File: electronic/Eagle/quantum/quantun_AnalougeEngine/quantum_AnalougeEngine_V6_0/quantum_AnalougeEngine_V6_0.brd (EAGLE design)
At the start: 210 x 70 mm, 281 parts, among them IC1 OP275, IC10 STM32F767ZIT6, IC11 PGA2320IDW, IC12 ESDA6V1BC6, IC13 USBLC6-4SC6, IC16 OP275, IC17 AD7606BSTZ-6, IC2 DAC084S085CIMM_NOPB, IC4 OP275, IC6 LAN8742A-CZ-TR, IC8 OP275, IC9 NE5532, J1 GWLEX-SMT-S988G_Y, K1 Relay, K2 Relay, K3 Relay, K4 Relay, K5 Relay, K6 Relay, K7 Relay, K8 Relay, T1 H1102NL, U1 78*_SMD, U12 ULN2003, U4 THAT1240, U6 THAT1240, U7 THAT1240, U8 THAT1240, Y1 NX3215SA-32.768K-STD-MUA-8, Y2 NX3225GD-8MHZ-STD-CRA-3, Y3 ABLS2-25.000MHZ-D4YF-T

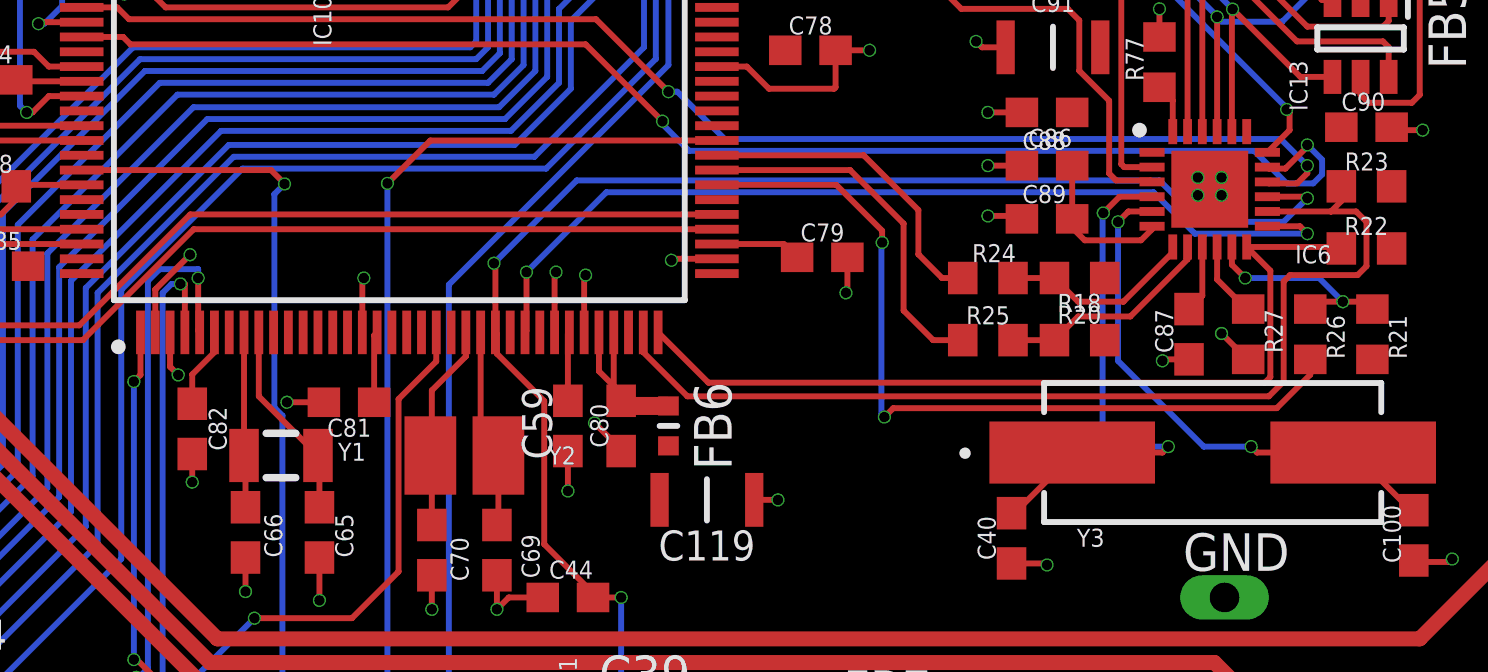
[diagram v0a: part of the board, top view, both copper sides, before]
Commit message: AnaloougeEngine_V6_0 & PSU_V2_3
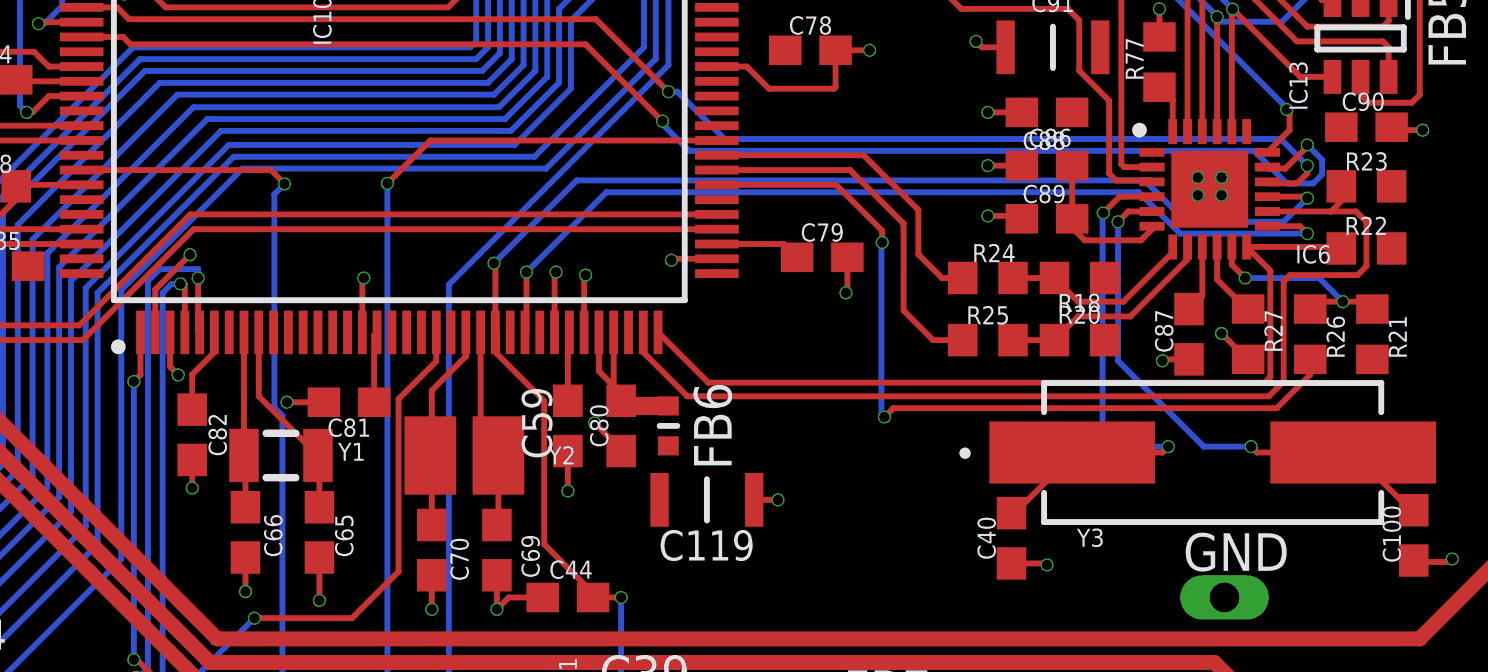
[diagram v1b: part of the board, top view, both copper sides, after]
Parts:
- moved C82 0.20 mm to (155.0, 20.3)
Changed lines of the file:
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@@
 <setting verticaltext="up"/>
 </settings>
-<grid distance="1" unitdist="mm" unit="mm" style="lines" multiple="1" display="yes" altdistance="0.000123031496" altunitdist="mil" altunit="mil"/>
+<grid distance="0.1" unitdist="mm" unit="mm" style="lines" multiple="1" display="yes" altdistance="0.000123031496" altunitdist="mil" altunit="mil"/>
 <layers>
 <layer number="1" name="Top(V+/+3V3)" color="59" fill="1" visible="yes" active="yes"/>
@@
 <attribute name="VALUE" x="159.665" y="19.495" size="1.016" layer="27"/>
 </element>
-<element name="C82" library="passive components" library_urn="urn:adsk.eagle:library:16365137" package="C0603" package3d_urn="urn:adsk.eagle:package:576738/3" value="100 nF" x="155" y="20.5" smashed="yes" rot="R90">
-<attribute name="NAME" x="156.165" y="19.765" size="0.6096" layer="25" rot="R90"/>
-<attribute name="VALUE" x="156.905" y="19.865" size="1.016" layer="27" rot="R90"/>
+<element name="C82" library="passive components" library_urn="urn:adsk.eagle:library:16365137" package="C0603" package3d_urn="urn:adsk.eagle:package:576738/3" value="100 nF" x="155" y="20.3" smashed="yes" rot="R90">
+<attribute name="NAME" x="156.165" y="19.565" size="0.6096" layer="25" rot="R90"/>
+<attribute name="VALUE" x="156.905" y="19.665" size="1.016" layer="27" rot="R90"/>
 </element>
 <element name="C83" library="passive components" library_urn="urn:adsk.eagle:library:16365137" package="C0603" package3d_urn="urn:adsk.eagle:package:576738/3" value="100 nF" x="147.9" y="39.1" smashed="yes" rot="R180">
@@
 <wire x1="159.45" y1="21.4" x2="158.2" y2="21.4" width="0.2" layer="1"/>
 <via x="158.2" y="21.4" extent="1-16" drill="0.35"/>
-<wire x1="155" y1="19.65" x2="155" y2="18.7" width="0.2" layer="1"/>
-<via x="155" y="18.7" extent="1-16" drill="0.35"/>
+<wire x1="155" y1="19.45" x2="155" y2="18.5" width="0.2" layer="1"/>
+<via x="155" y="18.5" extent="1-16" drill="0.35"/>
 <wire x1="156.8" y1="16.15" x2="156.8" y2="15" width="0.2" layer="1"/>
 <via x="156.8" y="15" extent="1-16" drill="0.35"/>
@@
 <wire x1="165.25" y1="26.05" x2="165.25" y2="23.762" width="0.2" layer="1"/>
 <wire x1="192.7" y1="28.3" x2="191.9" y2="27.5" width="0.2" layer="16"/>
-<wire x1="191.9" y1="27.5" x2="189.1" y2="27.5" width="0.2" layer="16"/>
-<wire x1="189.1" y1="27.5" x2="187.7" y2="28.9" width="0.2" layer="16"/>
-<wire x1="187.7" y1="28.9" x2="168" y2="28.9" width="0.2" layer="16"/>
+<wire x1="191.9" y1="27.5" x2="188.6" y2="27.5" width="0.2" layer="16"/>
+<wire x1="188.6" y1="27.5" x2="187.2" y2="28.9" width="0.2" layer="16"/>
+<wire x1="187.2" y1="28.9" x2="168" y2="28.9" width="0.2" layer="16"/>
 <wire x1="168.55" y1="14.8" x2="168.7" y2="14.8" width="0.2" layer="1"/>
 <via x="169.5" y="14.8" extent="1-16" drill="0.35"/>
@@
 <wire x1="192.45" y1="27.35" x2="192.7" y2="27.1" width="0.2" layer="1"/>
 <via x="192.7" y="27.1" extent="1-16" drill="0.35"/>
-<wire x1="192.7" y1="27.1" x2="188.9" y2="27.1" width="0.2" layer="16"/>
-<wire x1="188.9" y1="27.1" x2="187.5" y2="28.5" width="0.2" layer="16"/>
-<wire x1="187.5" y1="28.5" x2="169" y2="28.5" width="0.2" layer="16"/>
+<wire x1="192.7" y1="27.1" x2="188.4" y2="27.1" width="0.2" layer="16"/>
+<wire x1="188.4" y1="27.1" x2="187" y2="28.5" width="0.2" layer="16"/>
+<wire x1="187" y1="28.5" x2="169" y2="28.5" width="0.2" layer="16"/>
 <wire x1="169" y1="28.5" x2="166.3" y2="25.8" width="0.2" layer="16"/>
 <via x="166.3" y="25.8" extent="1-16" drill="0.35"/>
@@
 <contactref element="C59" pad="2"/>
 <contactref element="C119" pad="2"/>
-<wire x1="155" y1="21.35" x2="155" y2="22.34165625" width="0.2" layer="1"/>
+<wire x1="155" y1="21.15" x2="155" y2="22.34165625" width="0.2" layer="1"/>
 <wire x1="155" y1="22.34165625" x2="155.75" y2="23.09165625" width="0.2" layer="1"/>
 <wire x1="155.75" y1="23.09165625" x2="155.75" y2="23.762" width="0.2" layer="1"/>
@@
 <contactref element="C89" pad="2"/>
 <contactref element="C88" pad="2"/>
-<wire x1="187.45" y1="27.35" x2="187.45" y2="27.24895625" width="0.2" layer="1"/>
-<wire x1="187.45" y1="27.24895625" x2="187.07604375" y2="26.875" width="0.2" layer="1"/>
+<wire x1="187.45" y1="27.35" x2="187.500521875" y2="27.299478125" width="0.2" layer="1"/>
+<wire x1="187.500521875" y1="27.299478125" x2="187.07604375" y2="26.875" width="0.2" layer="1"/>
 <wire x1="187.07604375" y1="26.875" x2="185.175" y2="26.875" width="0.2" layer="1"/>
 <wire x1="185.175" y1="26.875" x2="184.75" y2="27.3" width="0.2" layer="1"/>
